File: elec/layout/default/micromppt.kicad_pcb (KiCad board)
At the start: 2 copper layers, 25.9 x 15.3 mm, 16 parts

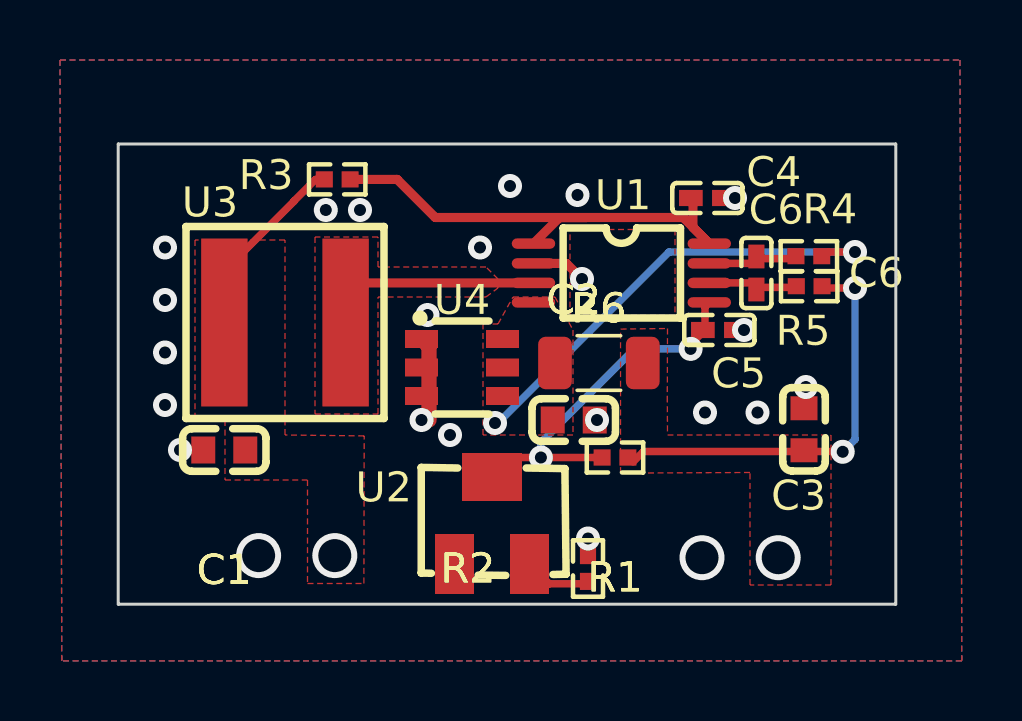
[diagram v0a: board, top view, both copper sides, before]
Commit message: v3 update
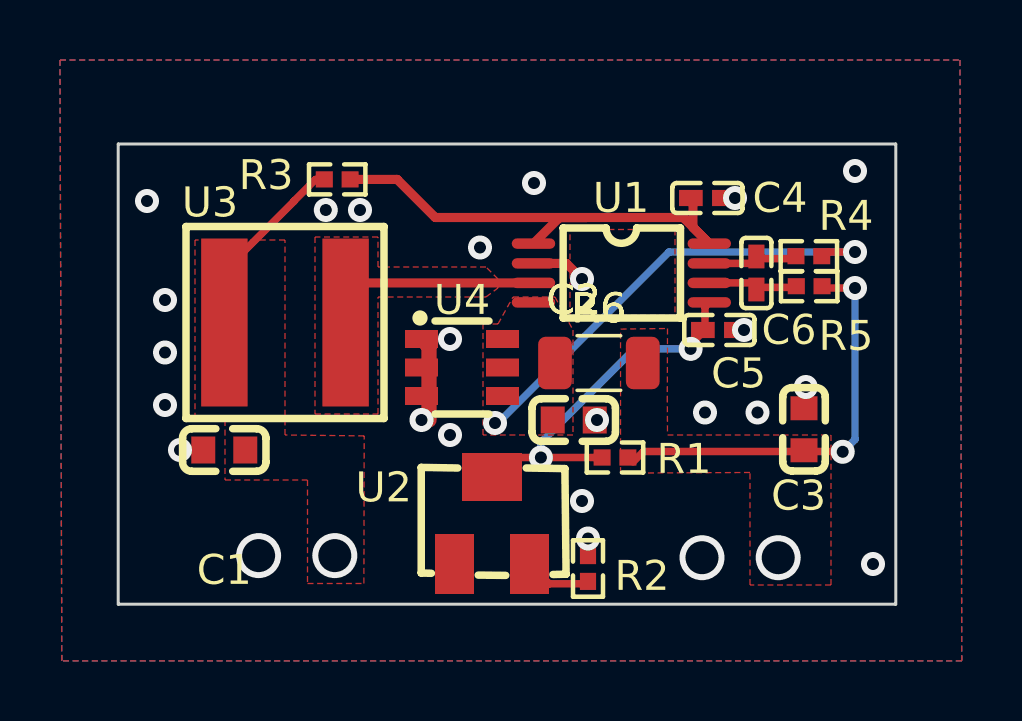
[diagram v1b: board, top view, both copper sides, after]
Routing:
- net gnd: vias 23 -> 25
